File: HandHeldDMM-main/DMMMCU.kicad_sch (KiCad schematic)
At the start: 23 parts, among them IC1 REF35300QDBVR, J1 Conn_02x03_Odd_Even, J3 Conn_01x03, J4 Conn_02x05_Odd_Even, SW1 SW_Push, U7 STM32F373CCTx, Y1 16Mhz

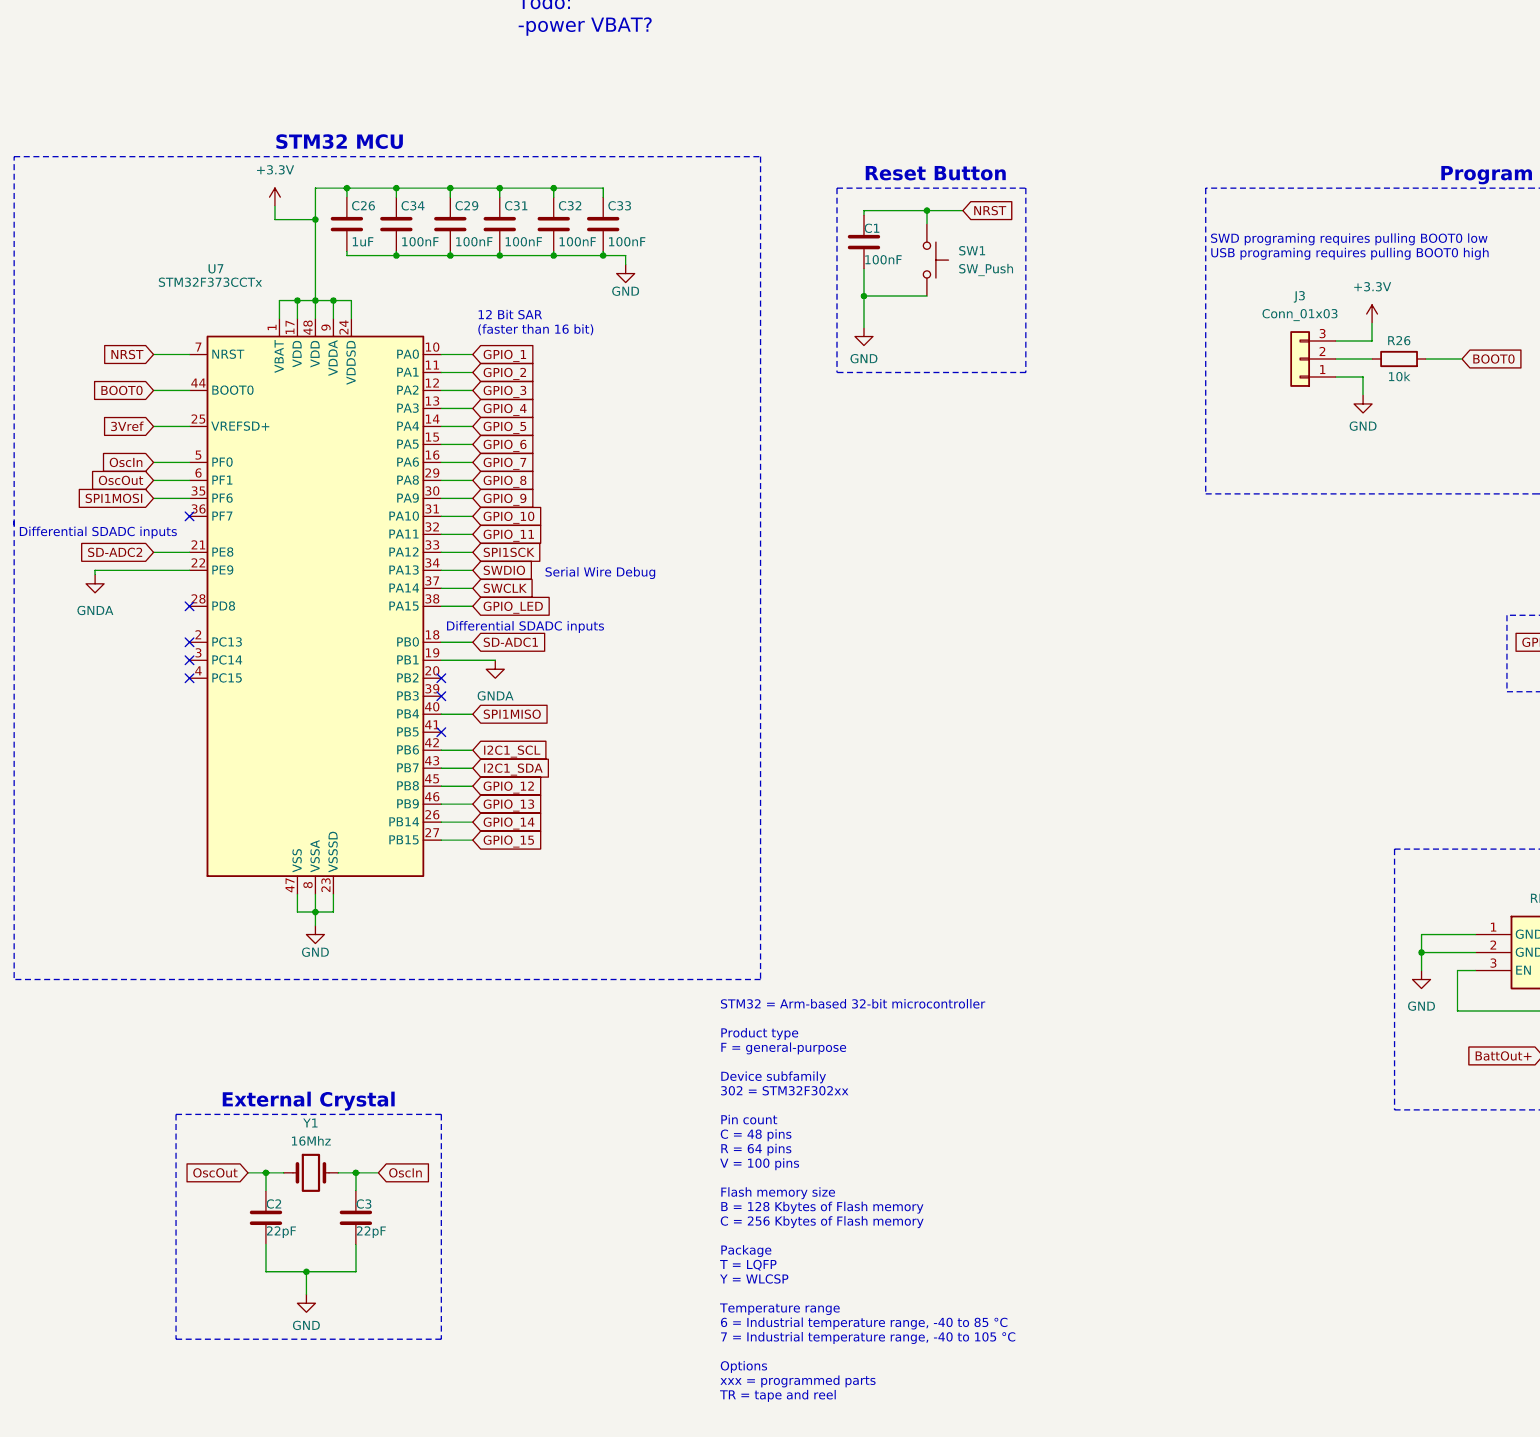
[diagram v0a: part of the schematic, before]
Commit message: PCB rev 1 with schematic change ideas
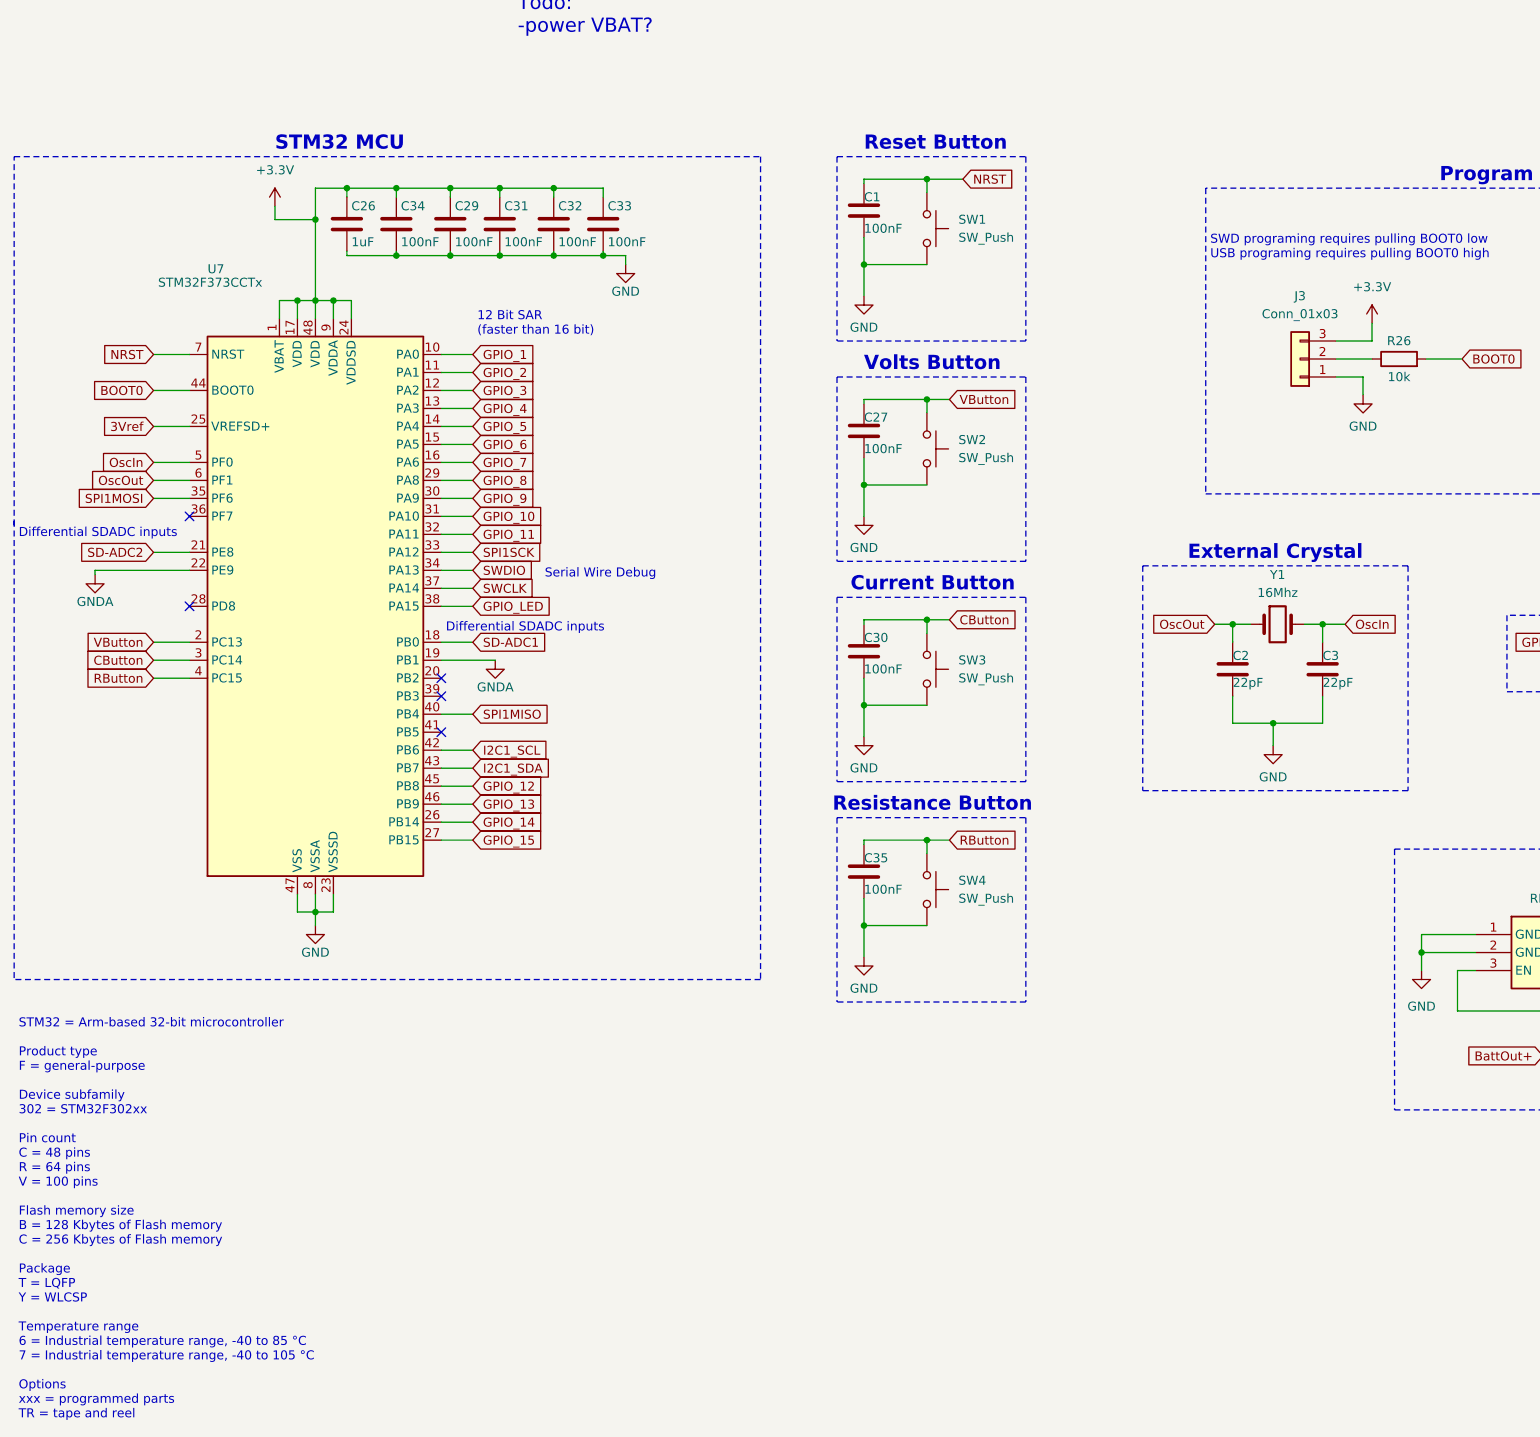
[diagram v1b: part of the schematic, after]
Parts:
- added C27, C30, C35: 100nF, Capacitor_SMD:C_0402_1005Metric_Pad0.74x0.62mm_HandSolder, symbol Device:C
- added SW2, SW3, SW4: SW_Push, Button_Switch_SMD:SW_SPST_B3S-1000, symbol Switch:SW_Push
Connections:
- net GND: now also C27.2, C30.2, C35.2, SW2.2, SW3.2, SW4.2
- net VButton: now reaches U7.2 (PC13)
- net VButton: now also C27.1, SW2.1
- net CButton: now reaches U7.3 (PC14)
- net CButton: now also C30.1, SW3.1
- net RButton: now reaches U7.4 (PC15)
- net RButton: now also C35.1, SW4.1
- no-connect marks 10 -> 7
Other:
- note added: "Current Button"
- note added: "Resistance Button"
- note added: "Volts Button"
- moved on the sheet: C1, C2, C3, SW1, Y1

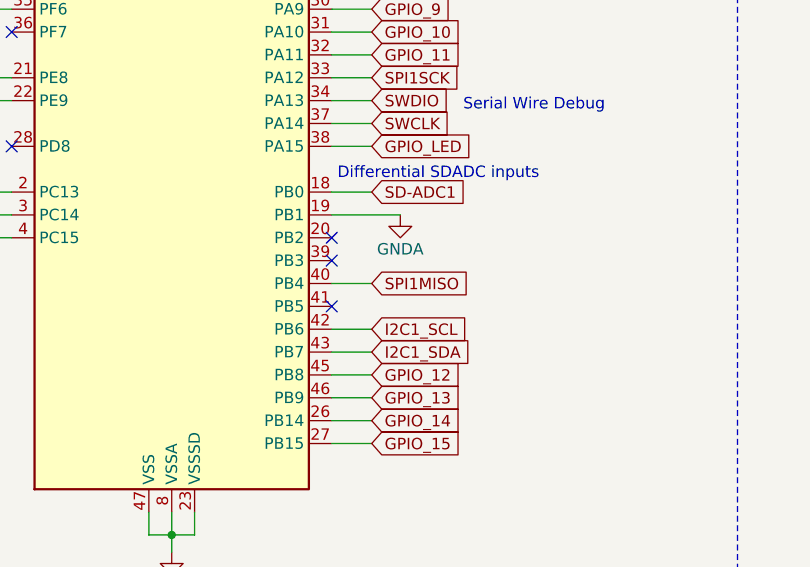
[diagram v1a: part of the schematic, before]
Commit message: Its going
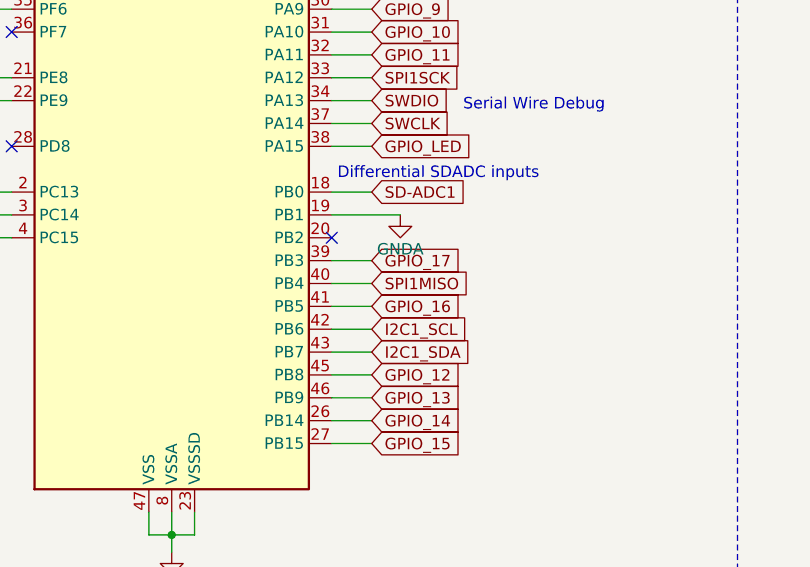
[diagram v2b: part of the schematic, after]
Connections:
- net GPIO_17: now reaches U7.39 (PB3)
- net GPIO_16: now reaches U7.41 (PB5)
- no-connect marks 7 -> 5
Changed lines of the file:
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@@
   (junction (at 69.215 31.115) (diameter 0) (color 0 0 0 0)
   )
-  (no_connect (at 75.565 93.345))
-  (no_connect (at 75.565 98.425))
   (no_connect (at 75.565 90.805))
   (no_connect (at 259.715 36.83))
@@
     (stroke (width 0) (type default))
   )
+  (wire (pts (xy 75.565 93.345) (xy 80.01 93.345))
+    (stroke (width 0) (type default))
+  )
   (wire (pts (xy 55.245 37.465) (xy 55.245 40.005))
     (stroke (width 0) (type default))
@@
   )
   (wire (pts (xy 75.565 73.025) (xy 80.01 73.025))
+    (stroke (width 0) (type default))
+  )
+  (wire (pts (xy 75.565 98.425) (xy 80.01 98.425))
     (stroke (width 0) (type default))
   )
@@
     )
   )
+  (global_label "GPIO_17" (shape input) (at 80.01 93.345 0) (fields_autoplaced)
+    (effects (font (size 1.27 1.27)) (justify left))
+    (property "Intersheetrefs" "${INTERSHEET_REFS}" (at 90.8571 93.345 0)
+      (effects (font (size 1.27 1.27)) (justify left) hide)
+    )
+  )
+  (global_label "GPIO_16" (shape input) (at 80.01 98.425 0) (fields_autoplaced)
+    (effects (font (size 1.27 1.27)) (justify left))
+    (property "Intersheetrefs" "${INTERSHEET_REFS}" (at 90.8571 98.425 0)
+      (effects (font (size 1.27 1.27)) (justify left) hide)
+    )
+  )
